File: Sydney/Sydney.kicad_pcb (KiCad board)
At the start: 2 copper layers, 99.1 x 54 mm, 6 parts, among them J1 Conn_01x02_Pin, U1 NT3H2111W0FHKH

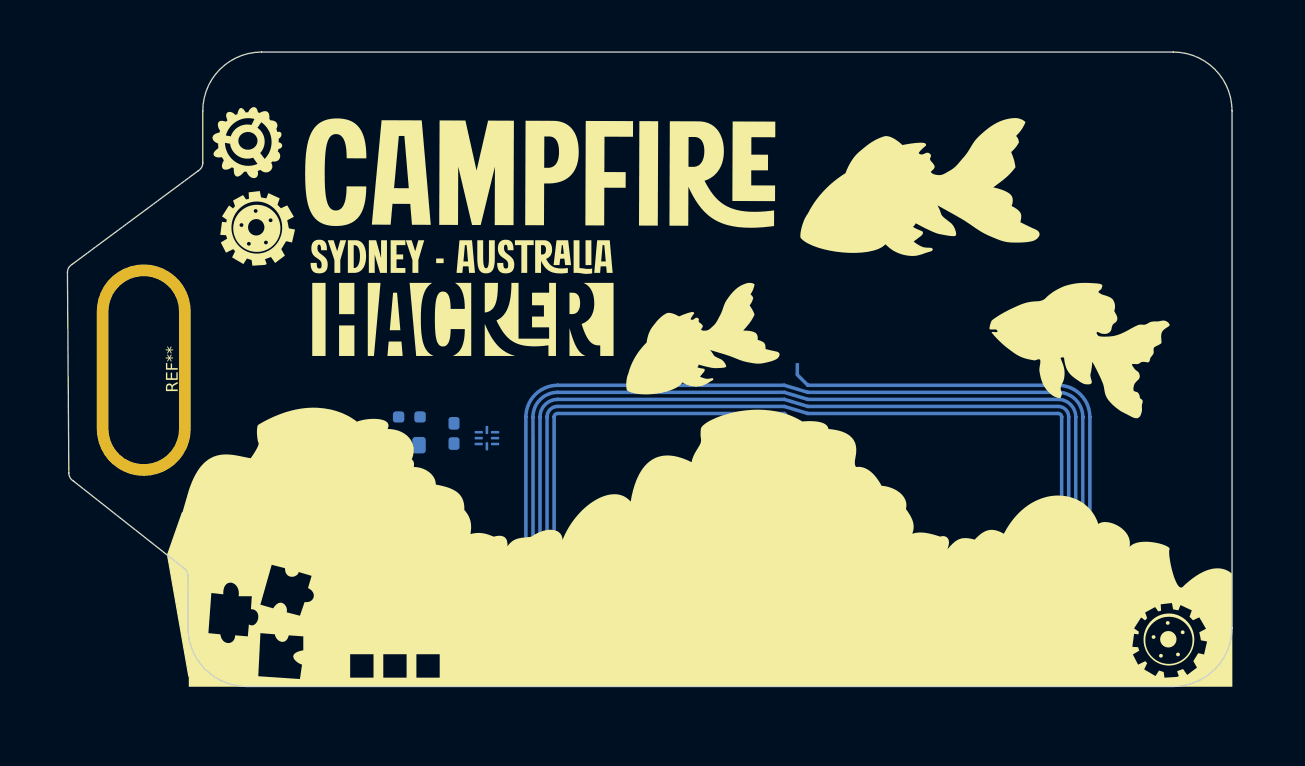
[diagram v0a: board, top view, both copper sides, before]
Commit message: finally works ish
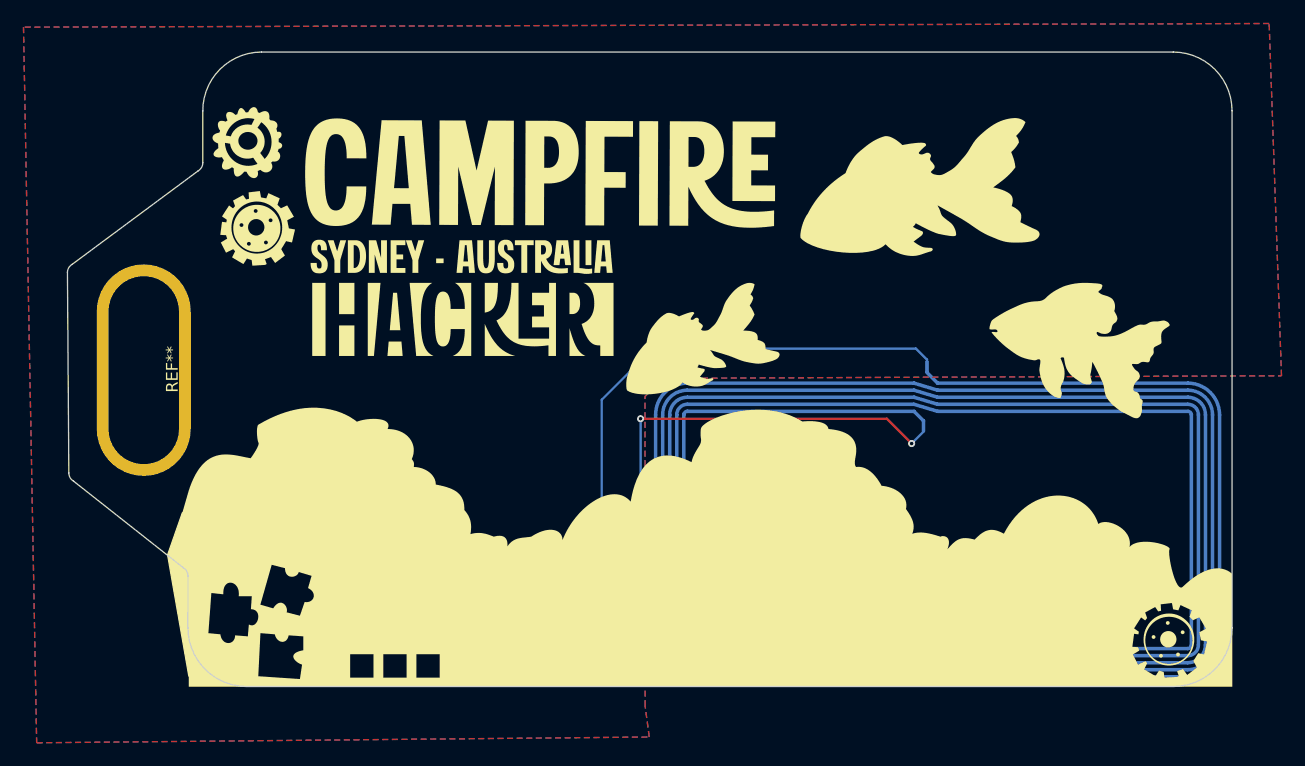
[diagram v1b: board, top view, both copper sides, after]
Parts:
- moved C1 17.7 mm to (197.0, 94.2)
- moved D1 17.7 mm to (193.0, 95.2)
- moved U1 17.7 mm to (199.8, 94.6)
- moved R1 17.7 mm to (193.2, 92.8)
- moved J1 11.0 mm to (228.3, 87.7)
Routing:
- net Net-(J1-Pin_1): track 0.00 -> 47.5 mm
- net Net-(J1-Pin_2): track 0.00 -> 42.6 mm, vias 0 -> 2
- net Net-(D1-K): track 0.00 -> 9.60 mm
- net Net-(U1-VCC): track 0.00 -> 6.13 mm
- net Net-(D1-A): track 0.00 -> 2.53 mm
- added copper zone on B.Cu, net (none)
- added copper zone on F.Cu, net (none)
